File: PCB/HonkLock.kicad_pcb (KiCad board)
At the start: 2 copper layers, 55.9 x 30.5 mm, 9 parts, among them J1 Conn_01x03_Pin, J2 Conn_01x06_Pin, J3 Conn_01x04_Pin, U1 Waveshare_ESP32_S3_Zero

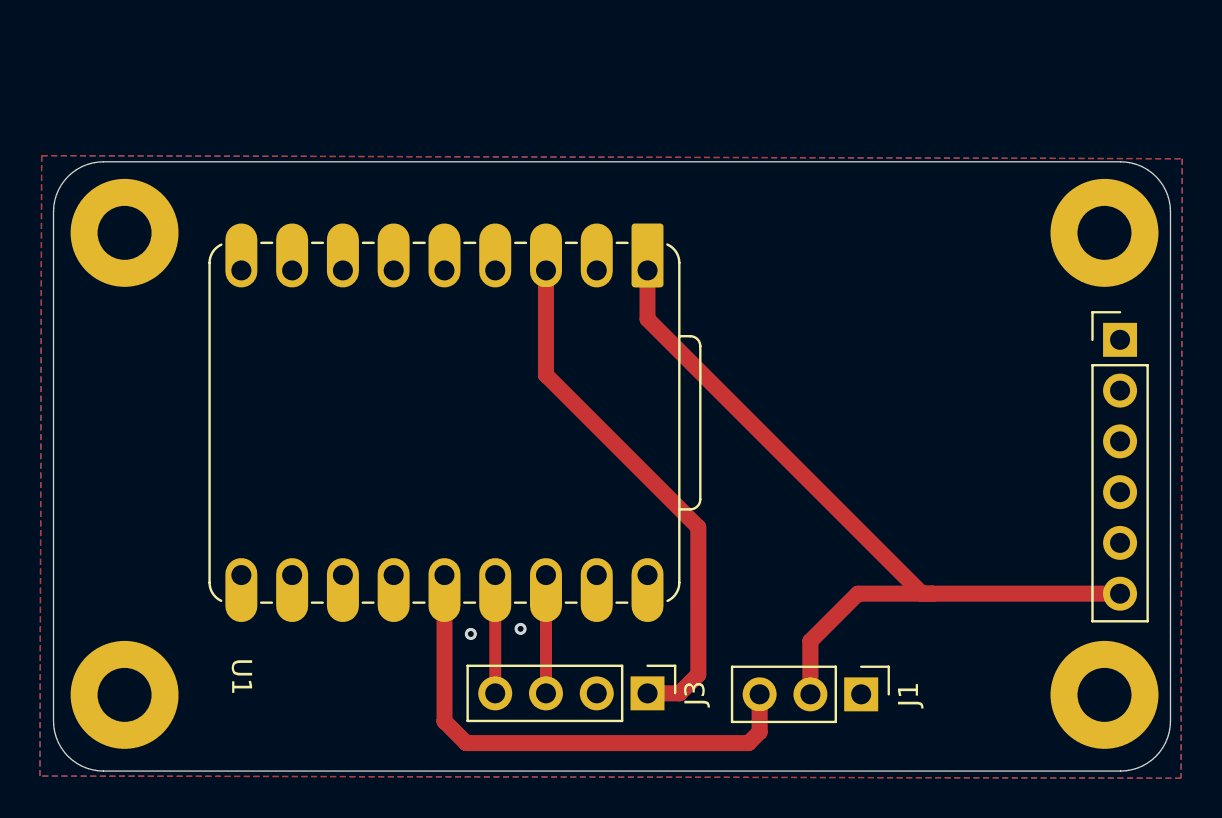
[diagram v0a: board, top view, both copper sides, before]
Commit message: Carrier board PCB
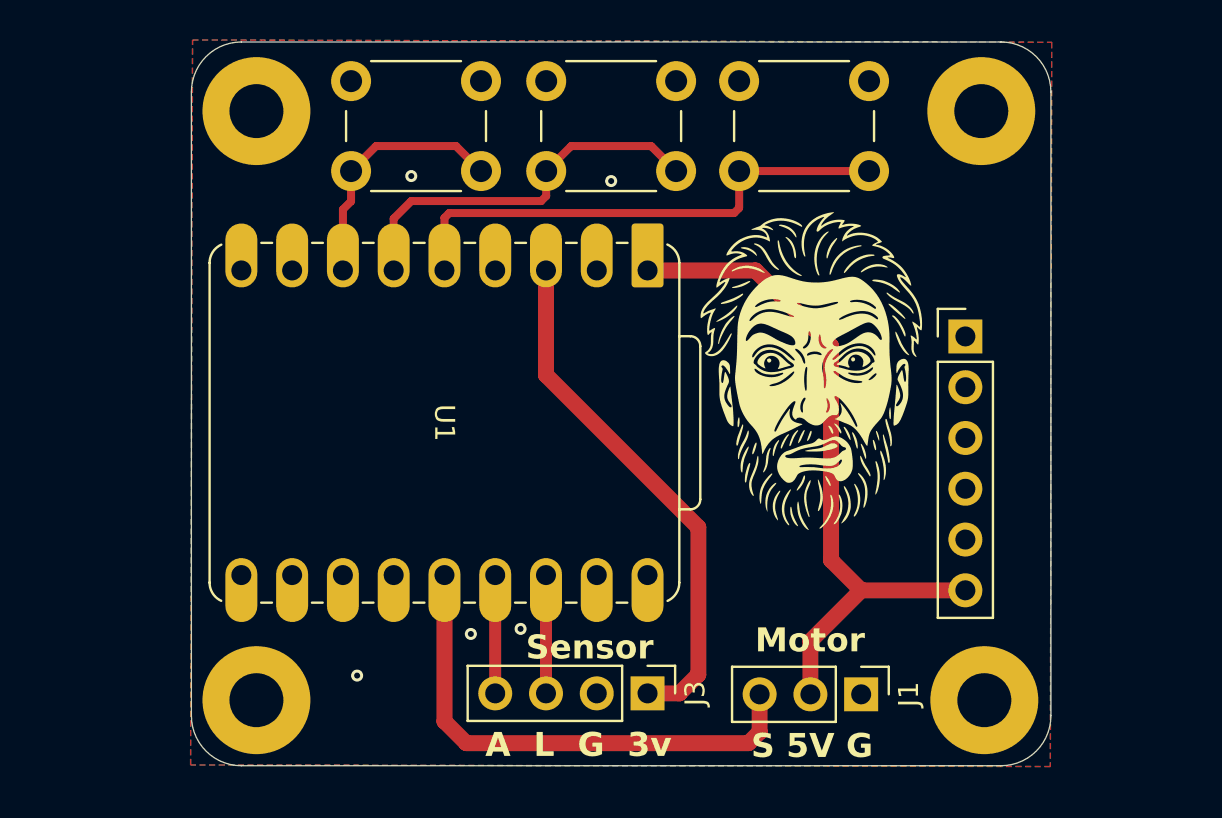
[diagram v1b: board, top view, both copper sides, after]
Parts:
- added SW1: SW_Push, Button_Switch_THT:SW_PUSH_6mm, F.Cu at (221.9, 66.2)
- added SW2: SW_Push, Button_Switch_THT:SW_PUSH_6mm, F.Cu at (212.2, 66.2)
- added SW3: SW_Push, Button_Switch_THT:SW_PUSH_6mm, F.Cu at (202.5, 66.2)
- moved H1 8.98 mm to (191.3, 63.2)
- moved H3 8.67 mm to (227.5, 63.2)
- moved G*** 7.88 mm to (206.5, 80.3)
- moved J2 7.74 mm to (226.7, 74.5)
- moved H2 6.60 mm to (191.3, 92.7)
- moved H4 6.02 mm to (227.7, 92.7)
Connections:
- U1 pad 5: unconnected-(U1-GP2-Pad5) -> Net-(U1-GP2)
- U1 pad 6: unconnected-(U1-GP3-Pad6) -> Net-(U1-GP3)
- U1 pad 7: unconnected-(U1-GP4-Pad7) -> Net-(U1-GP4)
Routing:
- net Net-(U1-GP2): track 0.00 -> 26.2 mm
- net Net-(U1-GP3): track 0.00 -> 19.5 mm
- net Net-(U1-GP4): track 0.00 -> 12.7 mm
- net VDD: track 41.5 -> 35.1 mm
- net unconnected-(U1-GP6-Pad9): track 0.00 -> 0.57 mm
- net unconnected-(U1-GP5-Pad8): track 0.00 -> 0.57 mm
- net GND: vias 2 -> 5
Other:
- board size 55.9 x 30.5 mm -> 43 x 36.2 mm
- board text added: "A L G 3v"
- board text added: "Motor"
- board text added: "S 5V G"
- board text added: "Sensor"
